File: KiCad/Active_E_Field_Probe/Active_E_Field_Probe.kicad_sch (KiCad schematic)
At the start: 6 parts

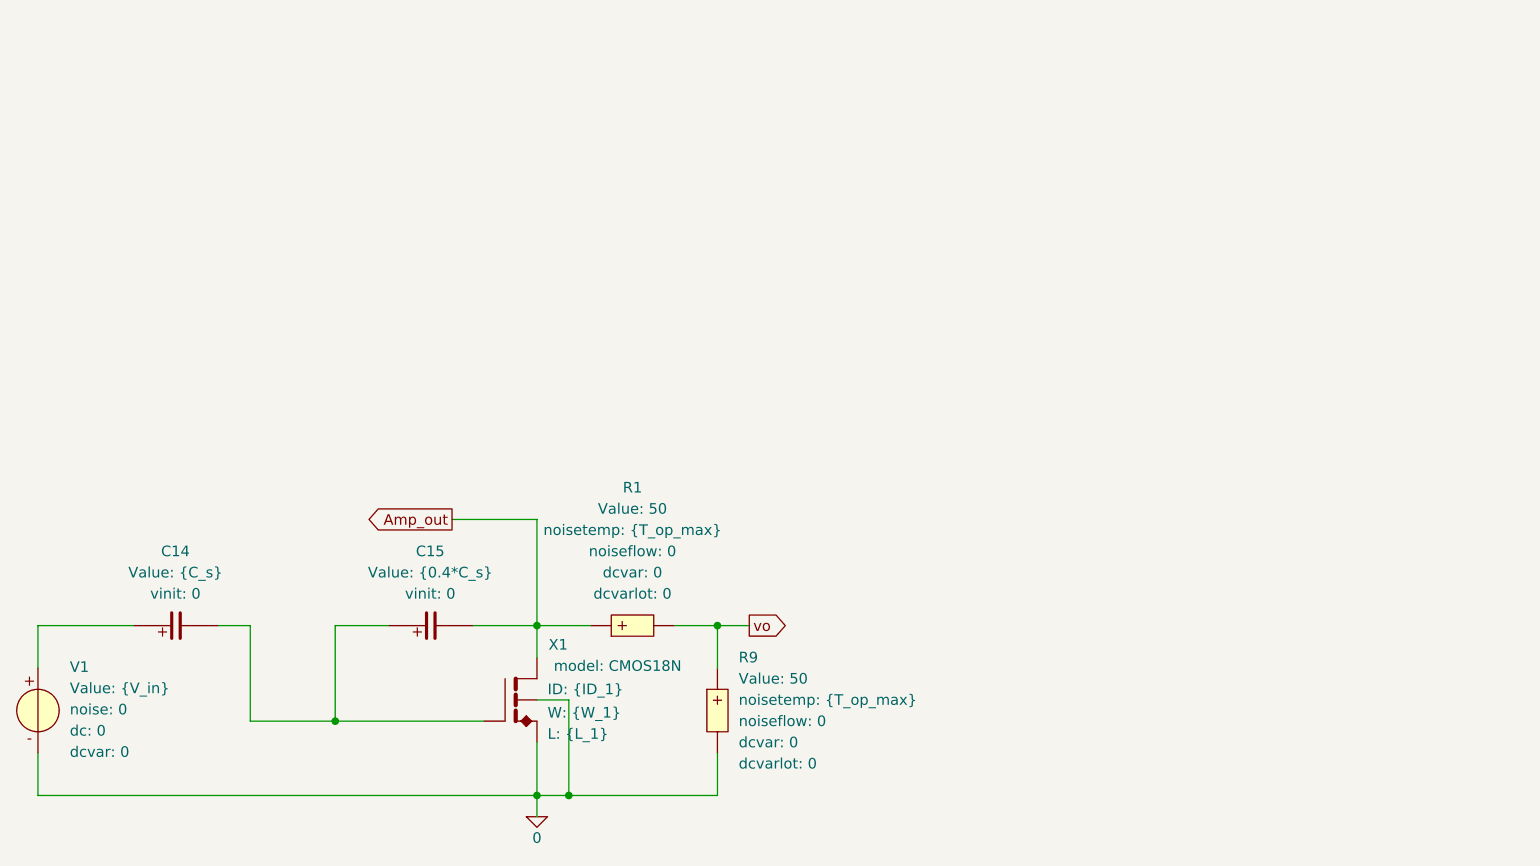
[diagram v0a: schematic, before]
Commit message: 2 stage
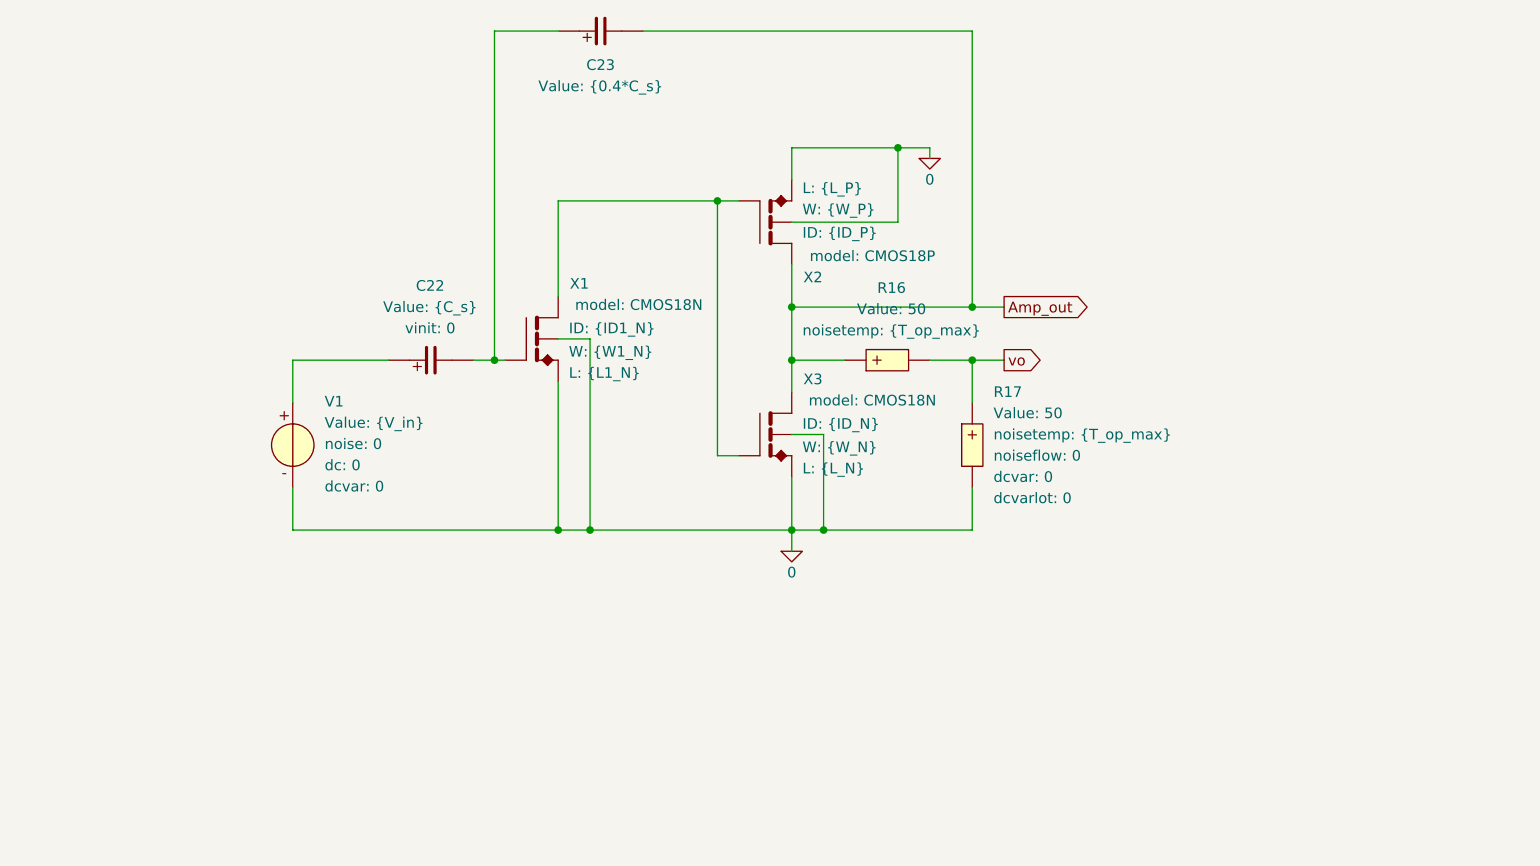
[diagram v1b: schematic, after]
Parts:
- removed C14: {C_s}, symbol SLiCAP:C
- removed C15: {0.4*C_s}, symbol SLiCAP:C
- removed R1, R9: 50, symbol SLiCAP:R
- added C22: {C_s}, symbol SLiCAP:C
- added C23: {0.4*C_s}, symbol SLiCAP:C
- added R16, R17: 50, symbol SLiCAP:R
- added X2, X3: ~, symbol SLiCAP:XM
- X1: ID {ID_1} -> {ID1_N}; L {L_1} -> {L1_N}; W {W_1} -> {W1_N}
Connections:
- net 0: now also R17.2, X2.3 (S), X2.4 (B), X3.3 (S), X3.4 (B)
- net Amp_out: now also C23.2, R16.1, X2.1 (D), X3.1 (D); no longer X1.1 (D)
- net vo: now also R16.2, R17.1
- net at X1.2 (G): now also C22.2, C23.1
- net at V1.1 (p): now also C22.1
- new net: X1.1 (D), X2.2 (G), X3.2 (G)

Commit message: something
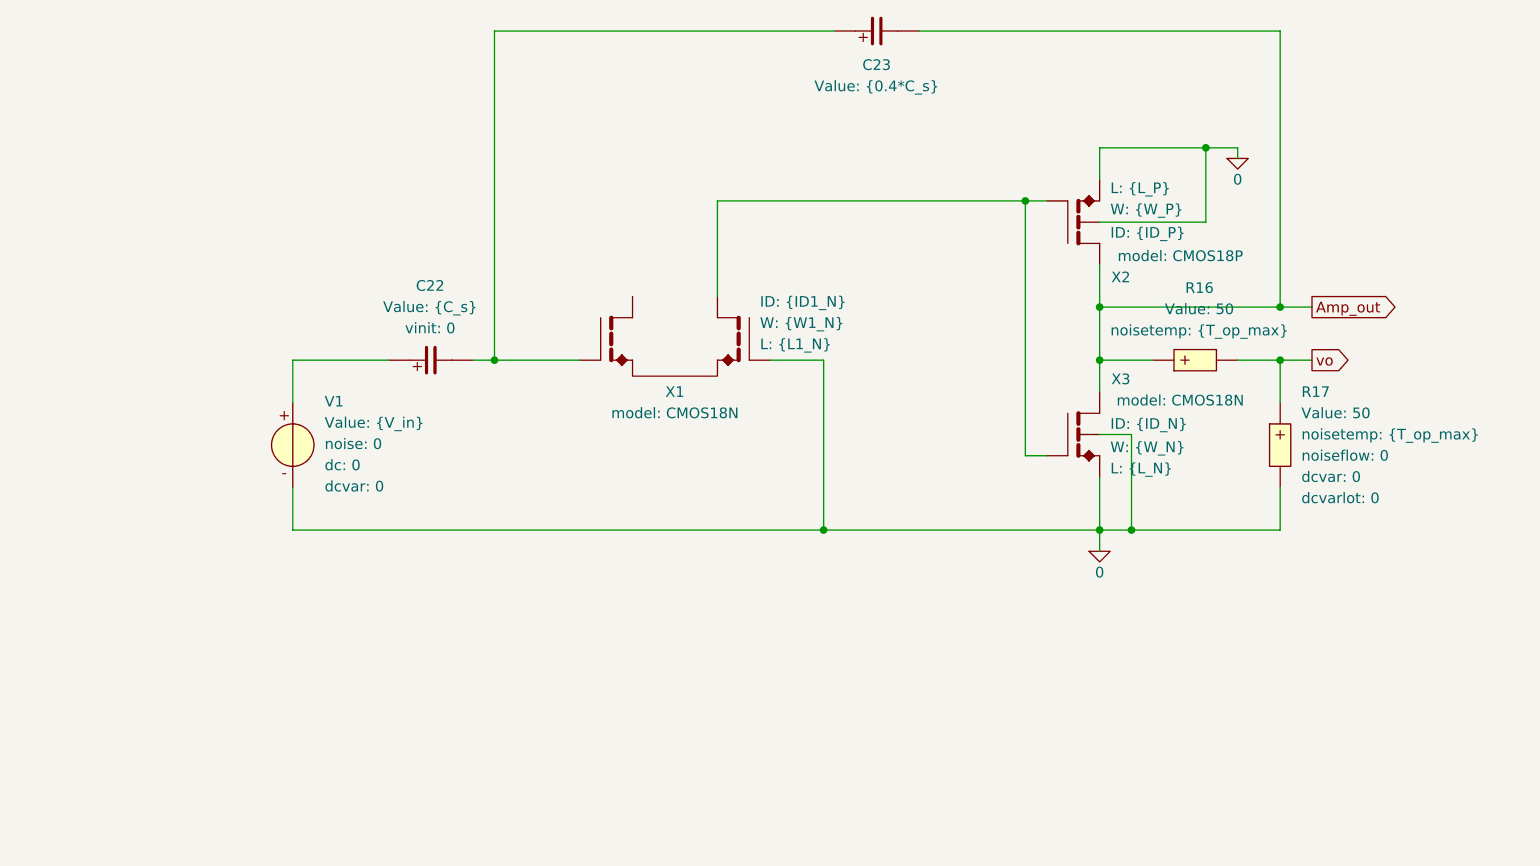
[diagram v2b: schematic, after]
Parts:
- removed X1: ~, symbol SLiCAP:XM
- added X1: ~, symbol SLiCAP:XMD
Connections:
- net 0: now also X1.4 (G2)
- net at C22.2, C23.1: now also X1.3 (G1)
- net at X2.2 (G), X3.2 (G): now also X1.2 (D2)
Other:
- moved on the sheet: C23, R16, R17, X2, X3
